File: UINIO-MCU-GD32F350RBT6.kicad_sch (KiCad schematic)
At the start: 21 parts

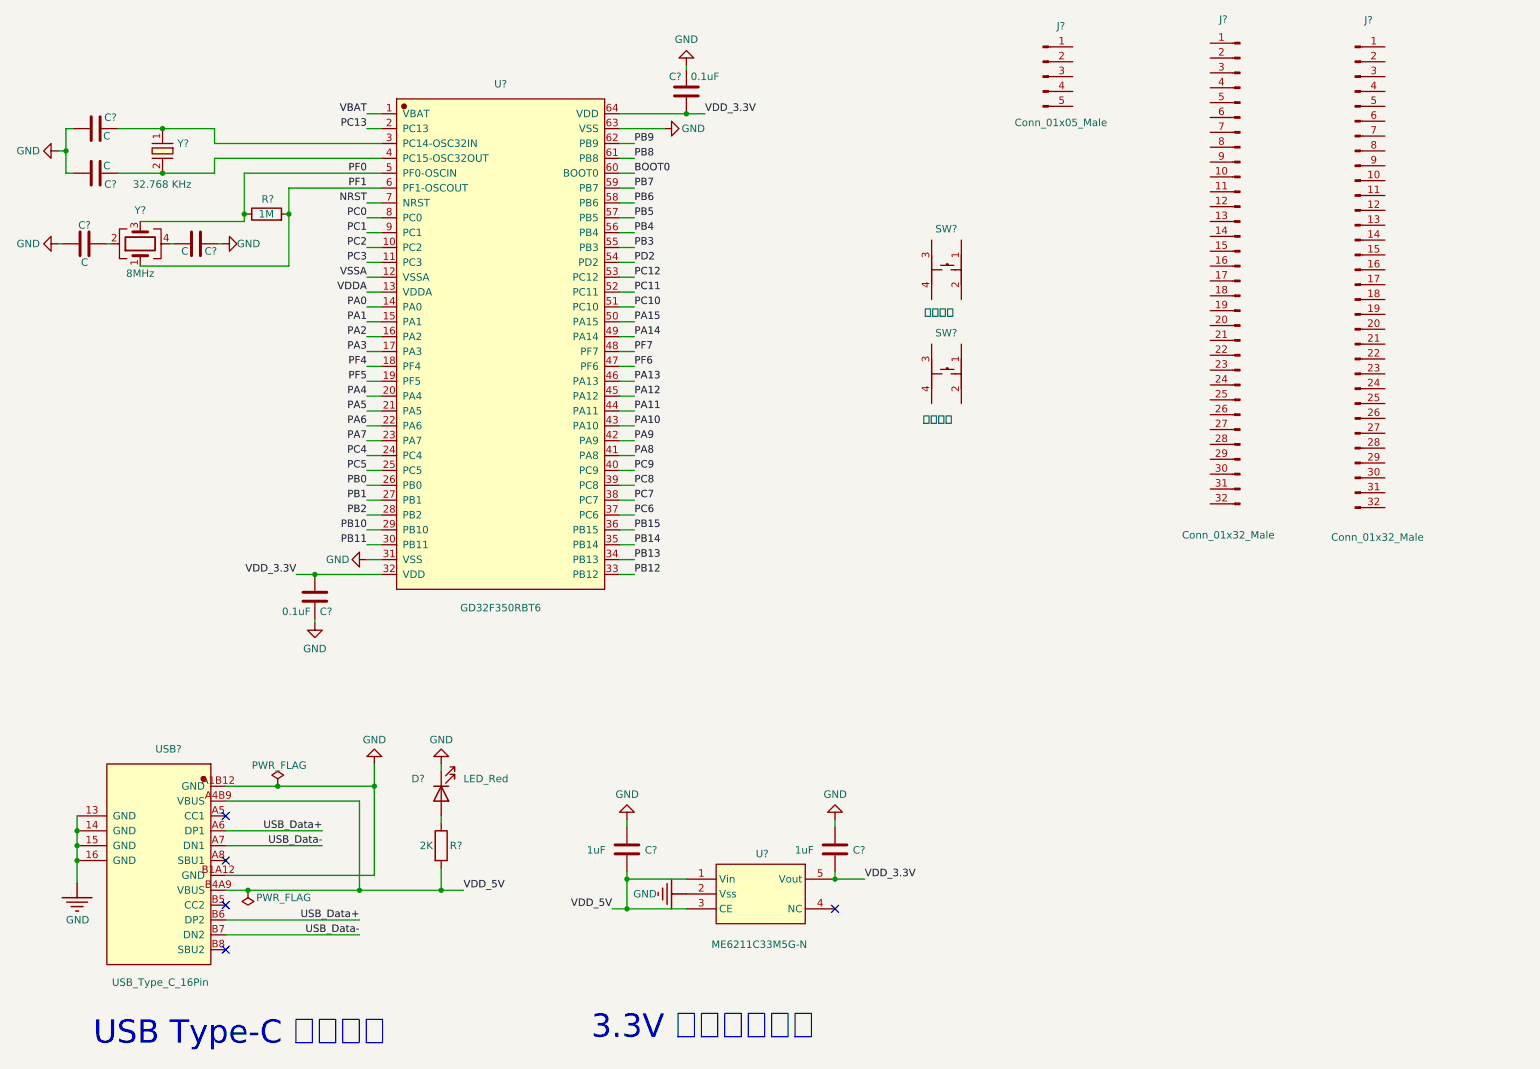
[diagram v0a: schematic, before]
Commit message: Update schematic diagram.
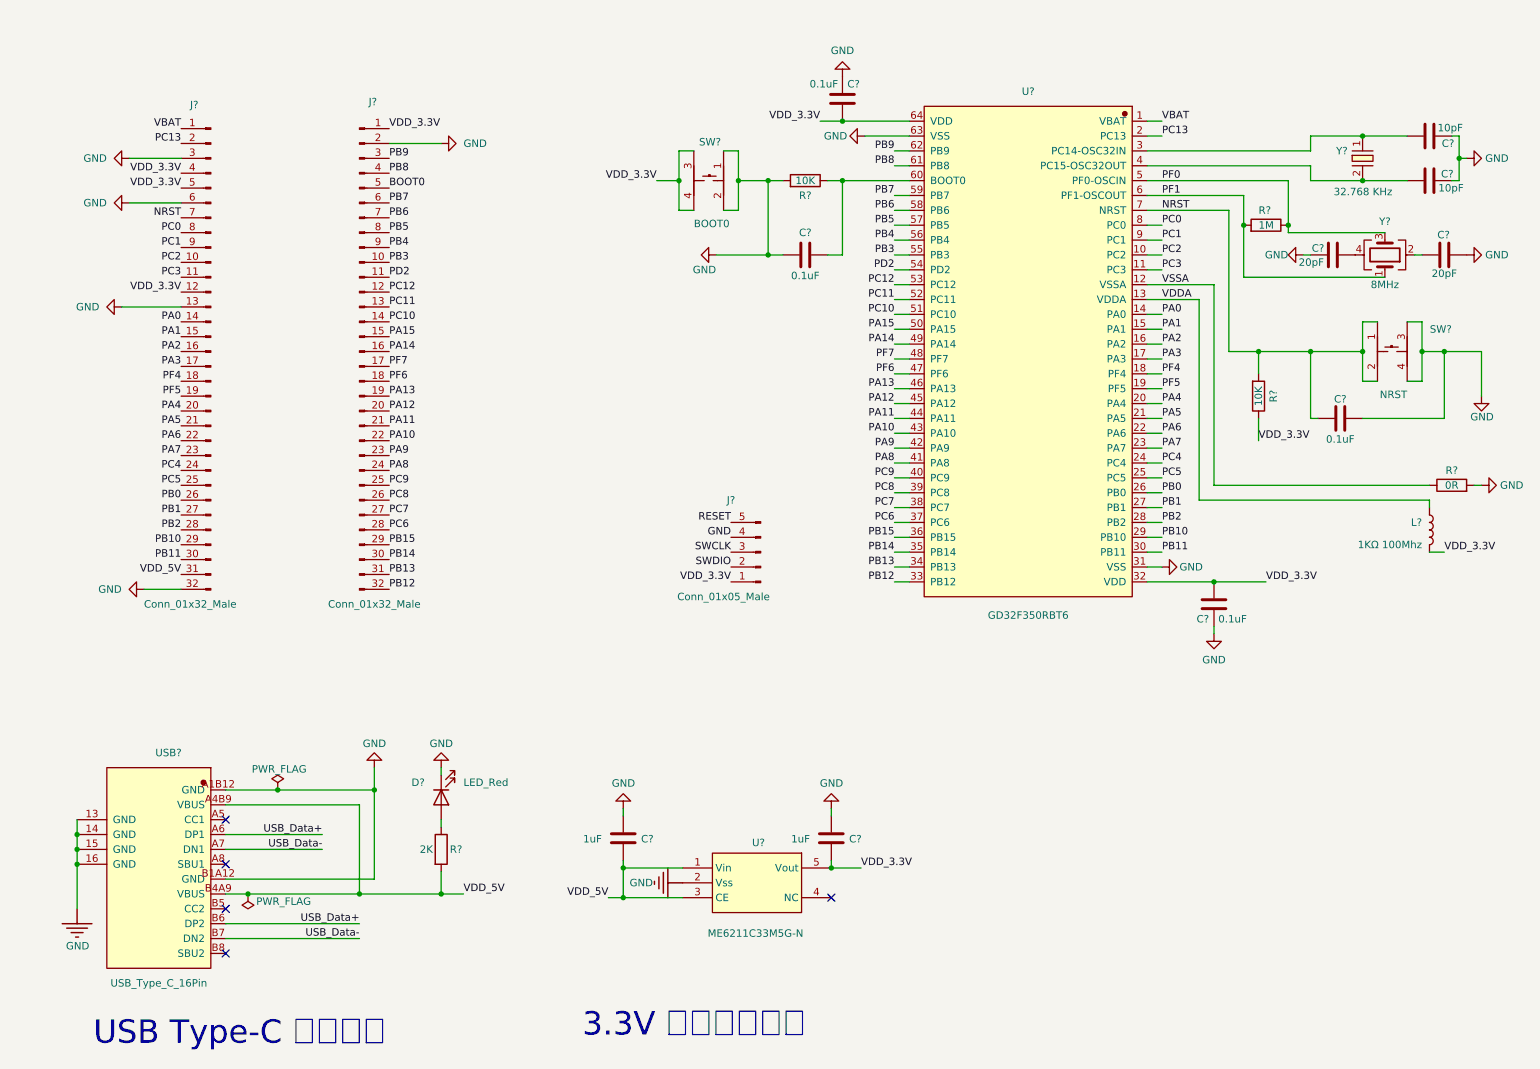
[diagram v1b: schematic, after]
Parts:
- removed SW?: 下载按键, Uinio:KEY-SMD_4P-L4.2-W3.4-P2.15-LS4.7, symbol Uinio:Key_YTS_A016S_1
- added C? (x2): 0.1uF, symbol Device:C
- added L?: 1KΩ 100Mhz, symbol Device:L
- added R? (x2): 10K, symbol Device:R
- added R?: 0R, symbol Device:R
- added SW?: BOOT0, Uinio:KEY-SMD_4P-L4.2-W3.4-P2.15-LS4.7, symbol Uinio:Key_YTS_A016S_1
- C? (x2): value C -> 10pF
- C? (x2): value C -> 20pF
- SW?: value 复位按键 -> NRST
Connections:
- net BOOT0: now also J?.5 (Pin_5); no longer U?.60 (BOOT0)
- net GND: now also J?.13 (Pin_13), J?.2 (Pin_2), J?.3 (Pin_3), J?.32 (Pin_32), J?.4 (Pin_4), J?.6 (Pin_6), SW?.3, SW?.4, C?.1, C?.2, R?.2, R?.2, SW?.1, SW?.2
- net NRST: now also J?.7 (Pin_7), SW?.1, SW?.2, C?.1, R?.2
- net PA0: now also J?.14 (Pin_14)
- net PA1: now also J?.15 (Pin_15)
- net PA10: now also J?.22 (Pin_22)
- net PA11: now also J?.21 (Pin_21)
- net PA12: now also J?.20 (Pin_20)
- net PA13: now also J?.19 (Pin_19)
- net PA14: now also J?.16 (Pin_16)
- net PA15: now also J?.15 (Pin_15)
- net PA2: now also J?.16 (Pin_16)
- net PA3: now also J?.17 (Pin_17)
- net PA4: now also J?.20 (Pin_20)
- net PA5: now also J?.21 (Pin_21)
- net PA6: now also J?.22 (Pin_22)
- net PA7: now also J?.23 (Pin_23)
- net PA8: now also J?.24 (Pin_24)
- net PA9: now also J?.23 (Pin_23)
- net PB0: now also J?.26 (Pin_26)
- net PB1: now also J?.27 (Pin_27)
- net PB10: now also J?.29 (Pin_29)
- net PB11: now also J?.30 (Pin_30)
- net PB12: now also J?.32 (Pin_32)
- net PB13: now also J?.31 (Pin_31)
- net PB14: now also J?.30 (Pin_30)
- net PB15: now also J?.29 (Pin_29)
- net PB2: now also J?.28 (Pin_28)
- net PB3: now also J?.10 (Pin_10)
- net PB4: now also J?.9 (Pin_9)
- net PB5: now also J?.8 (Pin_8)
- net PB6: now also J?.7 (Pin_7)
- net PB7: now also J?.6 (Pin_6)
- net PB8: now also J?.4 (Pin_4)
- net PB9: now also J?.3 (Pin_3)
- net PC0: now also J?.8 (Pin_8)
- net PC1: now also J?.9 (Pin_9)
- net PC10: now also J?.14 (Pin_14)
- net PC11: now also J?.13 (Pin_13)
- net PC12: now also J?.12 (Pin_12)
- net PC13: now also J?.2 (Pin_2)
- net PC2: now also J?.10 (Pin_10)
- net PC3: now also J?.11 (Pin_11)
- net PC4: now also J?.24 (Pin_24)
- net PC5: now also J?.25 (Pin_25)
- net PC6: now also J?.28 (Pin_28)
- net PC7: now also J?.27 (Pin_27)
- net PC8: now also J?.26 (Pin_26)
- net PC9: now also J?.25 (Pin_25)
- net PD2: now also J?.11 (Pin_11)
- net PF4: now also J?.18 (Pin_18)
- net PF5: now also J?.19 (Pin_19)
- net PF6: now also J?.18 (Pin_18)
- net PF7: now also J?.17 (Pin_17)
- net VBAT: now also J?.1 (Pin_1)
- net VDDA: now also L?.2
- net VDD_3.3V: now also J?.1 (Pin_1), J?.1 (Pin_1), J?.12 (Pin_12), J?.4 (Pin_4), J?.5 (Pin_5), L?.1, R?.1, SW?.3, SW?.4
- net VDD_5V: now also J?.31 (Pin_31)
- net VSSA: now also R?.1
- net SWDIO: now reaches J?.2 (Pin_2)
- net SWCLK: now reaches J?.3 (Pin_3)
- net RESET: now reaches J?.5 (Pin_5)
- new net: C?.2, R?.1, U?.60 (BOOT0)
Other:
- moved on the sheet: C?, D?, J?, R?, SW?, U?, USB?, Y?
